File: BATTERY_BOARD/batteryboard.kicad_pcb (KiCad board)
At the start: 2 copper layers, 95.9 x 90.2 mm, 42 parts, among them J1 KEYSTONE-1042, J10 Screw_Terminal_01x02, J11 Screw_Terminal_01x02, J12 Screw_Terminal_01x01, J2 KEYSTONE-1042, J3 KEYSTONE-1042, J4 KEYSTONE-1042, J5 KEYSTONE-1042, J6 KEYSTONE-1042, J7 JST_PH_S2B-PH-SM4, J8 Screw_Terminal_01x02, J9 Screw_Terminal_01x02, Q1 IRF7458, Q2 IRF7458, U1 R5460N233AF

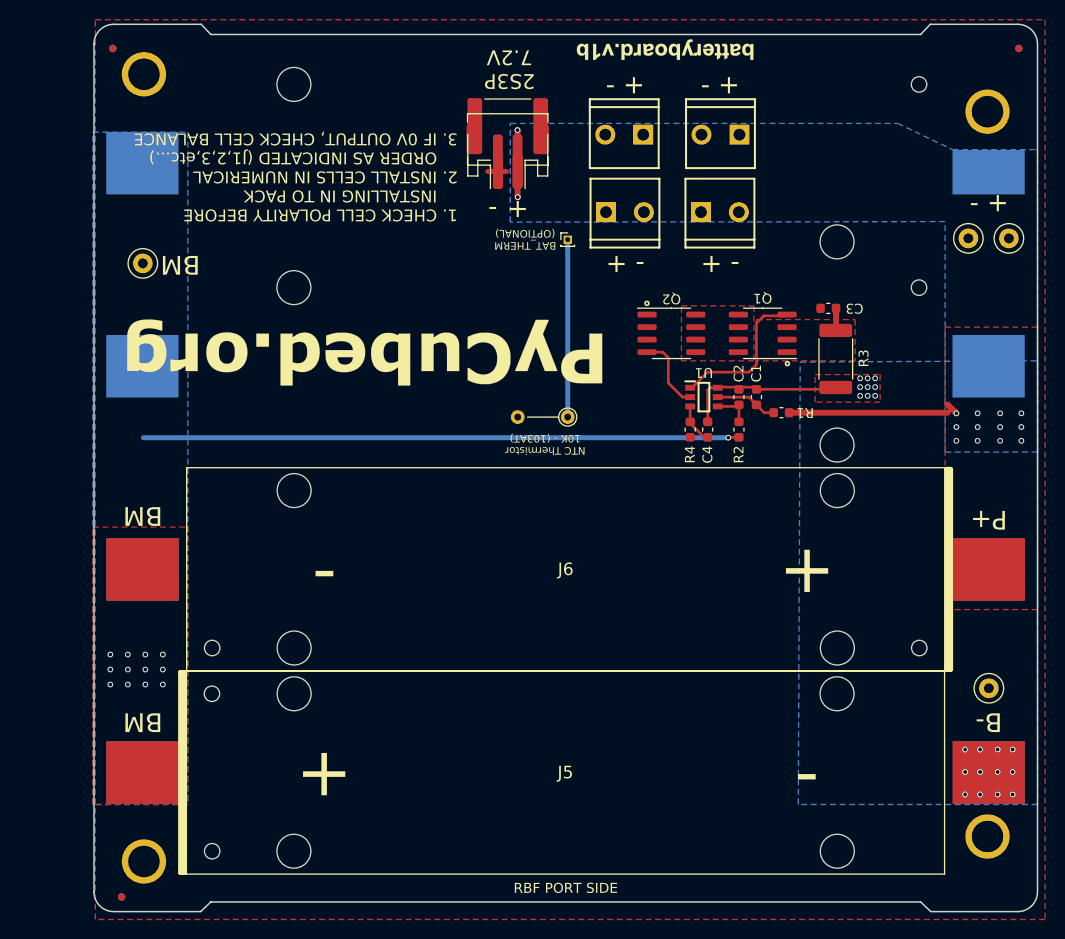
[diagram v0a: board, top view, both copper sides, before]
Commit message: Schematic Verified
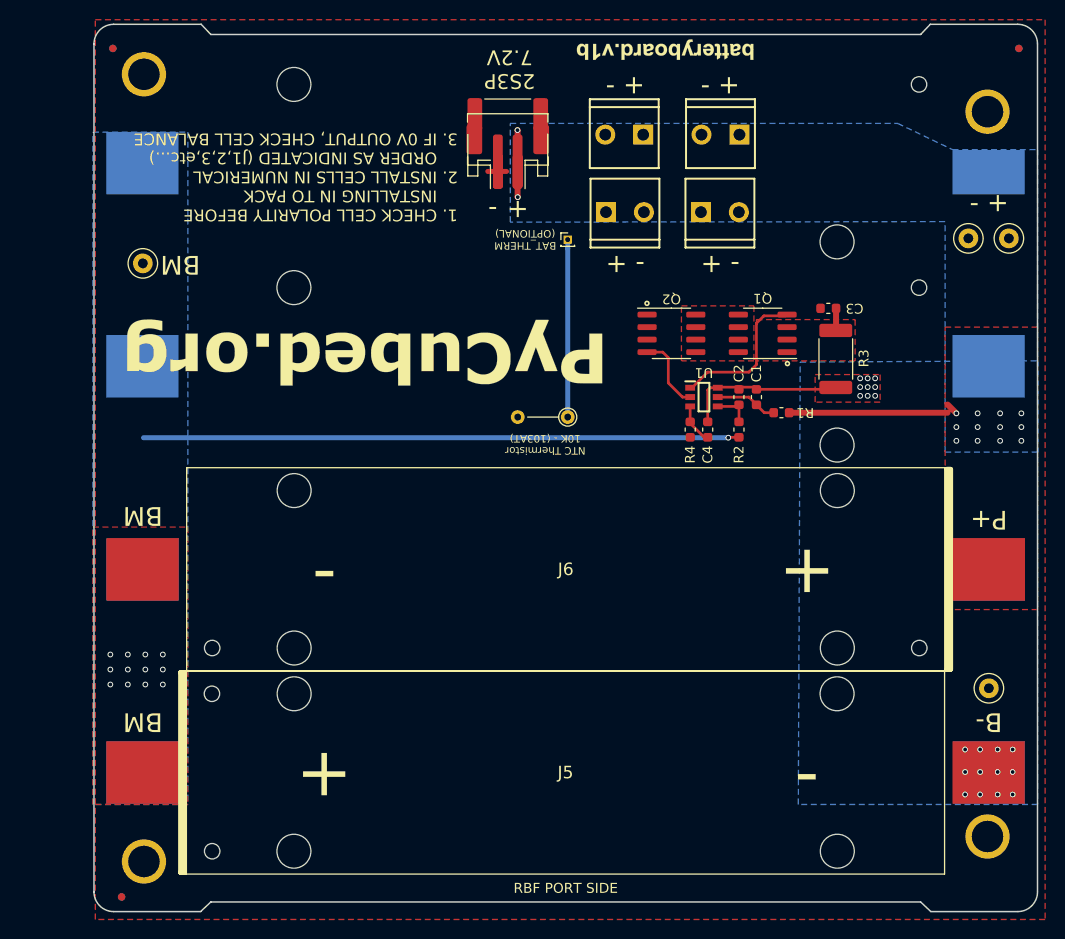
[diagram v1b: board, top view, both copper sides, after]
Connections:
- H1 pad 1: Net-(H1-Pad1) -> unconnected-(H1-Pad1)
- H2 pad 1: Net-(H2-Pad1) -> unconnected-(H2-Pad1)
- H3 pad 1: Net-(H3-Pad1) -> unconnected-(H3-Pad1)
- H4 pad 1: Net-(H4-Pad1) -> unconnected-(H4-Pad1)
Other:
- net class Default removed
